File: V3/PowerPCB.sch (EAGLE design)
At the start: 123 parts, among them CON1 PINHEAD_1X12-2.54-FEMALE, CON3 PINHEAD_1X08-2.54-FEMALE, CON4 PINHEAD_1X06-2.54-FEMALE, CON7 PINHEAD_1X06-2.54-FEMALE, IC1 TPS54560B, IC10 TPS54260, IC2 TPS54560B, IC3 TPS54560B, IC4 TPS54560B, IC5 INA169, J1 CONNECTION-7MM, M1 BATTERY_CON-XT30-RA, M2 BATTERY_CON-XT30-RA, M3 BATTERY_CON-XT30-RA, M4 BATTERY_CON-XT30-RA, M5 BATTERY_CON-XT30-RA, M6 BATTERY_CON-XT30-RA, M7 BATTERY_CON-XT30-RA, Q1 IRFR2407PBF, Q2 IRFR2407PBF, Q3 IRFR2407PBF

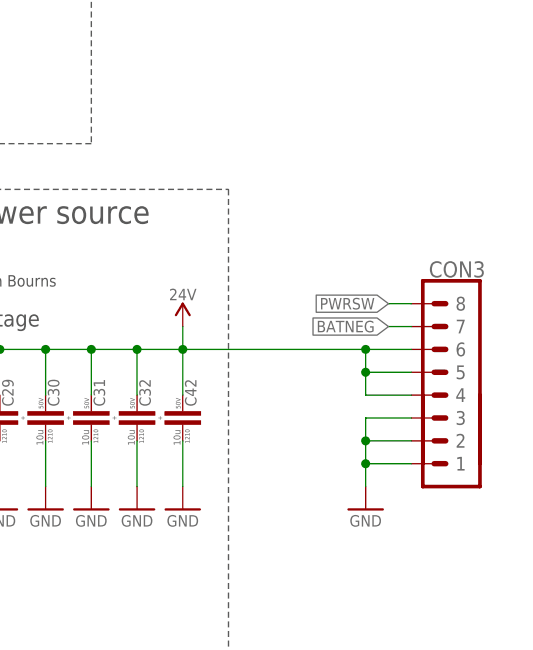
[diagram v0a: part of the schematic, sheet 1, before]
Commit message: V3 finalization
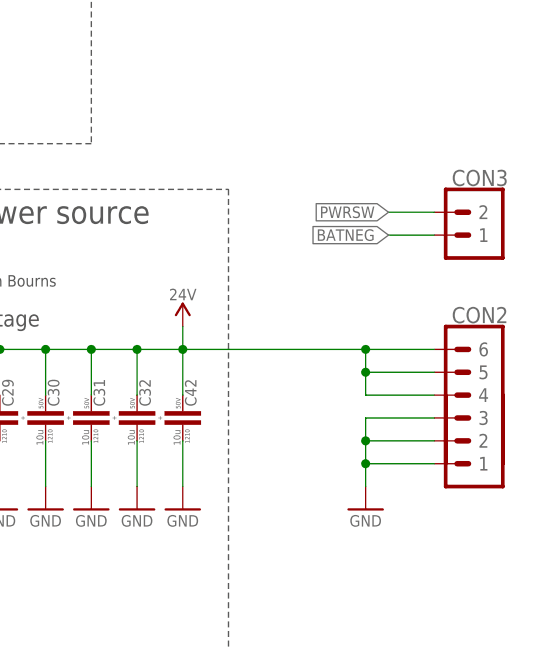
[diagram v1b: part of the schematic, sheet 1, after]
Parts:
- added CON2: PINHEAD_1X06-2.54-FEMALE, pinhead:PINHEAD_1X06-2.54-FEMALE
- CON3: value PINHEAD_1X08-2.54-FEMALE -> PINHEAD_1X02-2.54-FEMALE; device pinhead:PINHEAD_1X08-2.54-FEMALE -> pinhead:PINHEAD_1X02-2.54-FEMALE
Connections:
- net BATNEG: now also CON3.1; no longer CON3.7
- net GND: now also CON2.1, CON2.2, CON2.3; no longer CON3.1, CON3.2, CON3.3
- net PWRSW: now also CON3.2; no longer CON3.8
- net VDD_24V: now also CON2.4, CON2.5, CON2.6; no longer CON3.4, CON3.5, CON3.6
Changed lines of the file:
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@@
 <part name="+P4" library="supply_symbols" library_urn="urn:adsk.eagle:library:5017758" deviceset="VDC" device=""/>
 <part name="+P15" library="supply_symbols" library_urn="urn:adsk.eagle:library:5017758" deviceset="5VFMU" device=""/>
-<part name="CON3" library="pinhead" library_urn="urn:adsk.eagle:library:2540341" deviceset="PINHEAD_1X08" device="-2.54-FEMALE" package3d_urn="urn:adsk.eagle:package:7747001/3"/>
 <part name="U$1" library="supply_symbols" library_urn="urn:adsk.eagle:library:5017758" deviceset="BATNEG" device="" value="BATNEG"/>
 <part name="U$2" library="supply_symbols" library_urn="urn:adsk.eagle:library:5017758" deviceset="BATNEG" device="" value="BATNEG"/>
@@
 <part name="+P20" library="supply_symbols" library_urn="urn:adsk.eagle:library:5017758" deviceset="4V" device=""/>
 <part name="GND79" library="supply_symbols" library_urn="urn:adsk.eagle:library:5017758" deviceset="GND" device="" value="GND"/>
+<part name="CON2" library="pinhead" library_urn="urn:adsk.eagle:library:2540341" deviceset="PINHEAD_1X06" device="-2.54-FEMALE" package3d_urn="urn:adsk.eagle:package:15321847/2"/>
+<part name="CON3" library="pinhead" library_urn="urn:adsk.eagle:library:2540341" deviceset="PINHEAD_1X02" device="-2.54-FEMALE" package3d_urn="urn:adsk.eagle:package:32579456/2"/>
 </parts>
 <sheets>
@@
 <attribute name="VALUE" x="149.86" y="199.39" size="1.27" layer="97" font="vector" ratio="15" align="center"/>
 </instance>
-<instance part="CON3" gate="G$1" x="170.18" y="38.1" smashed="yes" rot="MR0">
-<attribute name="NAME" x="167.64" y="62.23" size="1.778" layer="95" font="vector" ratio="15" rot="MR0" align="center"/>
-</instance>
 <instance part="CON4" gate="G$1" x="160.02" y="182.88" smashed="yes" rot="R180">
 <attribute name="NAME" x="157.48" y="163.83" size="1.778" layer="95" font="vector" ratio="15" rot="R180" align="center"/>
@@
 <instance part="GND79" gate="1" x="160.02" y="213.36" smashed="yes" rot="MR0">
 <attribute name="VALUE" x="160.02" y="212.09" size="1.27" layer="96" font="vector" ratio="15" rot="MR0" align="center"/>
+</instance>
+<instance part="CON2" gate="G$1" x="172.72" y="38.1" smashed="yes" rot="MR0">
+<attribute name="NAME" x="170.18" y="57.15" size="1.778" layer="95" font="vector" ratio="15" rot="MR0" align="center"/>
+</instance>
+<instance part="CON3" gate="G$1" x="172.72" y="63.5" smashed="yes" rot="MR0">
+<attribute name="NAME" x="170.18" y="72.39" size="1.778" layer="95" font="vector" ratio="15" rot="MR0" align="center"/>
 </instance>
 </instances>
@@
 <pinref part="GND18" gate="1" pin="GND"/>
 <wire x1="157.48" y1="38.1" x2="157.48" y2="40.64" width="0.1524" layer="91"/>
-<wire x1="157.48" y1="40.64" x2="162.56" y2="40.64" width="0.1524" layer="91"/>
-<wire x1="162.56" y1="43.18" x2="157.48" y2="43.18" width="0.1524" layer="91"/>
+<wire x1="157.48" y1="40.64" x2="165.1" y2="40.64" width="0.1524" layer="91"/>
+<wire x1="165.1" y1="43.18" x2="157.48" y2="43.18" width="0.1524" layer="91"/>
 <wire x1="157.48" y1="43.18" x2="157.48" y2="40.64" width="0.1524" layer="91"/>
 <junction x="157.48" y="40.64"/>
-<wire x1="162.56" y1="45.72" x2="157.48" y2="45.72" width="0.1524" layer="91"/>
+<wire x1="165.1" y1="45.72" x2="157.48" y2="45.72" width="0.1524" layer="91"/>
 <wire x1="157.48" y1="45.72" x2="157.48" y2="43.18" width="0.1524" layer="91"/>
 <junction x="157.48" y="43.18"/>
-<pinref part="CON3" gate="G$1" pin="1"/>
-<pinref part="CON3" gate="G$1" pin="2"/>
-<pinref part="CON3" gate="G$1" pin="3"/>
+<pinref part="CON2" gate="G$1" pin="1"/>
+<pinref part="CON2" gate="G$1" pin="2"/>
+<pinref part="CON2" gate="G$1" pin="3"/>
 </segment>
 <segment>
@@
 <junction x="137.16" y="53.34"/>
 <wire x1="137.16" y1="53.34" x2="157.48" y2="53.34" width="0.1524" layer="91"/>
-<wire x1="157.48" y1="53.34" x2="162.56" y2="53.34" width="0.1524" layer="91"/>
-<wire x1="162.56" y1="50.8" x2="157.48" y2="50.8" width="0.1524" layer="91"/>
+<wire x1="157.48" y1="53.34" x2="165.1" y2="53.34" width="0.1524" layer="91"/>
+<wire x1="165.1" y1="50.8" x2="157.48" y2="50.8" width="0.1524" layer="91"/>
 <wire x1="157.48" y1="50.8" x2="157.48" y2="53.34" width="0.1524" layer="91"/>
 <junction x="157.48" y="53.34"/>
-<wire x1="162.56" y1="48.26" x2="157.48" y2="48.26" width="0.1524" layer="91"/>
+<wire x1="165.1" y1="48.26" x2="157.48" y2="48.26" width="0.1524" layer="91"/>
 <wire x1="157.48" y1="48.26" x2="157.48" y2="50.8" width="0.1524" layer="91"/>
 <junction x="157.48" y="50.8"/>
-<pinref part="CON3" gate="G$1" pin="4"/>
-<pinref part="CON3" gate="G$1" pin="5"/>
-<pinref part="CON3" gate="G$1" pin="6"/>
+<pinref part="CON2" gate="G$1" pin="4"/>
+<pinref part="CON2" gate="G$1" pin="5"/>
+<pinref part="CON2" gate="G$1" pin="6"/>
 </segment>
 </net>
@@
 <net name="PWRSW" class="0">
 <segment>
-<pinref part="CON3" gate="G$1" pin="8"/>
-<wire x1="162.56" y1="58.42" x2="160.02" y2="58.42" width="0.1524" layer="91"/>
-<label x="160.02" y="58.42" size="1.27" layer="95" rot="R180" xref="yes"/>
+<label x="160.02" y="68.58" size="1.27" layer="95" rot="R180" xref="yes"/>
+<pinref part="CON3" gate="G$1" pin="2"/>
+<wire x1="165.1" y1="68.58" x2="160.02" y2="68.58" width="0.1524" layer="91"/>
 </segment>
 </net>
 <net name="BATNEG" class="0">
 <segment>
-<pinref part="CON3" gate="G$1" pin="7"/>
-<wire x1="160.02" y1="55.88" x2="162.56" y2="55.88" width="0.1524" layer="91"/>
-<label x="160.02" y="55.88" size="1.27" layer="95" rot="R180" xref="yes"/>
-</segment>
-</net>
+<label x="160.02" y="66.04" size="1.27" layer="95" rot="R180" xref="yes"/>
+<pinref part="CON3" gate="G$1" pin="1"/>
+<wire x1="160.02" y1="66.04" x2="165.1" y2="66.04" width="0.1524" layer="91"/>
+</segment>
+</net>
